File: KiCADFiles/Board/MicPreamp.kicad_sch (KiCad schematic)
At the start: 13 parts, among them U302B2 OPA2348, U6 THAT151xx08

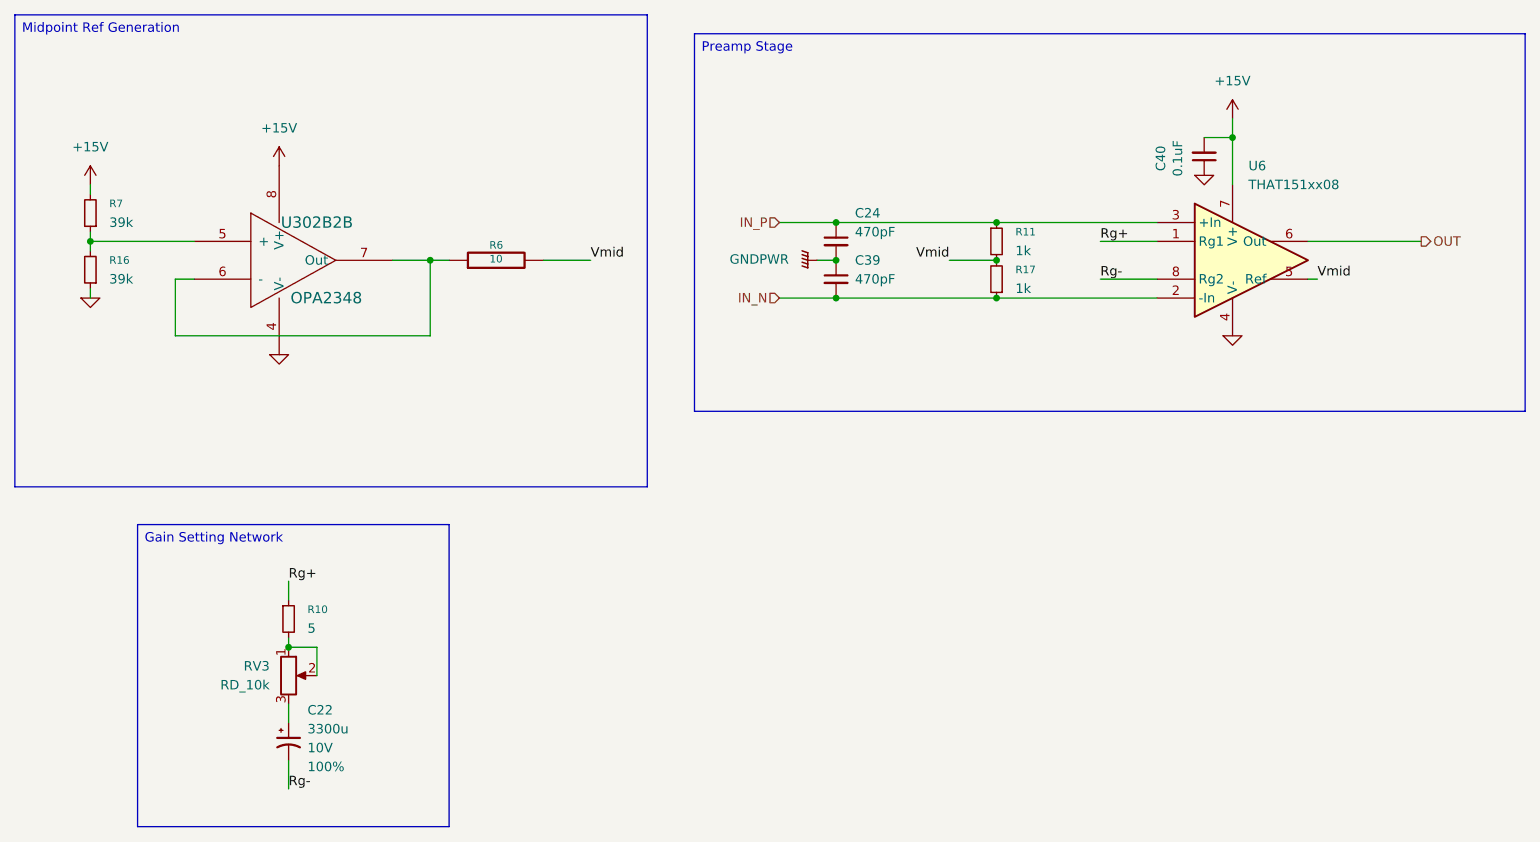
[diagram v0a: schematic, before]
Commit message: chose all components
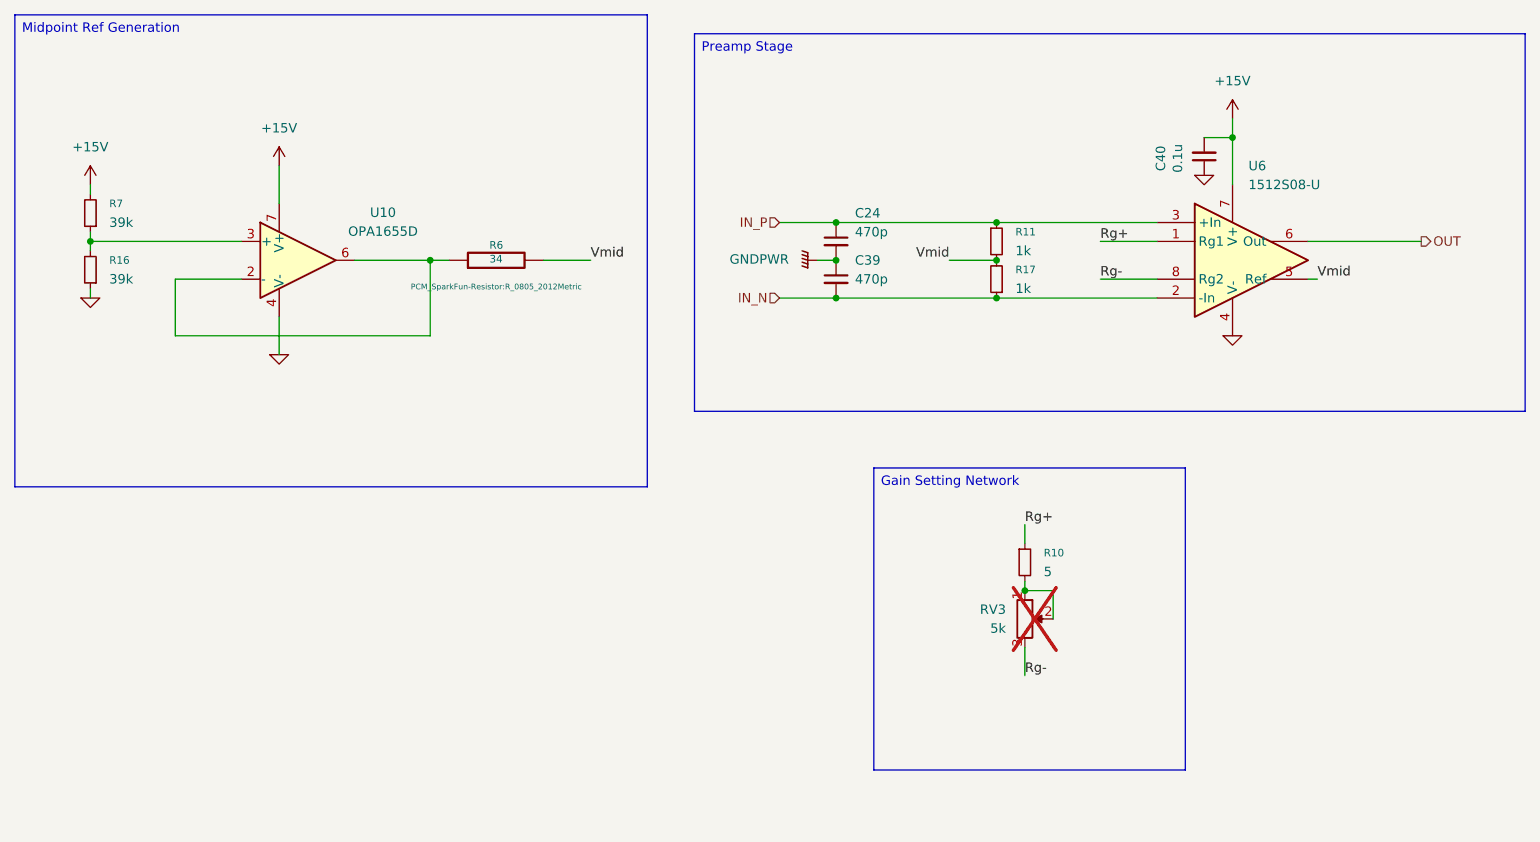
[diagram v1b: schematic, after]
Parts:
- removed C22: 3300u, ~, symbol PCM_SparkFun-Capacitor:C_Polarized_Small
- removed U302B2: OPA2348, symbol SuperAudioBoard-rescue:OPA2348
- added U10: OPA1655D, Package_SO:SOIC-8_3.9x4.9mm_P1.27mm, symbol Amplifier_Operational:OPA1655D
- C24, C39: value 470pF -> 470p; MPN (none) -> C0603C471J5GACTU
- C40: value 0.1uF -> 0.1u; MPN (none) -> CL10B104KB8NNNL
- R10: footprint (none) -> PCM_SparkFun-Resistor:R_0805_2012Metric; MPN (none) -> RC0805FR-074R7L
- R11, R17: footprint (none) -> PCM_SparkFun-Resistor:R_0805_2012Metric; MPN (none) -> ERA-6AEB102V
- R16, R7: footprint (none) -> PCM_SparkFun-Resistor:R_0805_2012Metric; MPN (none) -> ERA-6AEB3922V
- R6: value 10 -> 34; footprint ~ -> PCM_SparkFun-Resistor:R_0805_2012Metric; MPN (none) -> CRCW080534R0FKEA
- RV3: value RD_10k -> 5k; footprint (none) -> Potentiometer_THT:Potentiometer_Alps_RK163_Single_Horizontal; MPN (none) -> RV16AF-10-15K-C5K-3LA; now not fitted
- U6: value THAT151xx08 -> 1512S08-U; footprint (none) -> Package_SO:SOIC-8_5.3x5.3mm_P1.27mm; MPN (none) -> 1512S08-U
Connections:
- net +15V: now also U10.7 (V+)
- net GND: now also U10.4 (V-)
- net Rg-: now also RV3.3
- net at R6.1: now also U10.2 (-), U10.6
- net at R16.2, R7.1: now also U10.3 (+)
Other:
- moved on the sheet: R10
